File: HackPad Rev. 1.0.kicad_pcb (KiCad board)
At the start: 2 copper layers, 87 x 56.5 mm, 14 parts, among them SW1 SW_Push_45deg, SW2 SW_Push_45deg, SW3 SW_Push_45deg, SW4 SW_Push_45deg, SW5 RotaryEncoder_Switch, SW6 SW_Push_45deg, U1 Seeed Studio XIAO SAMD21

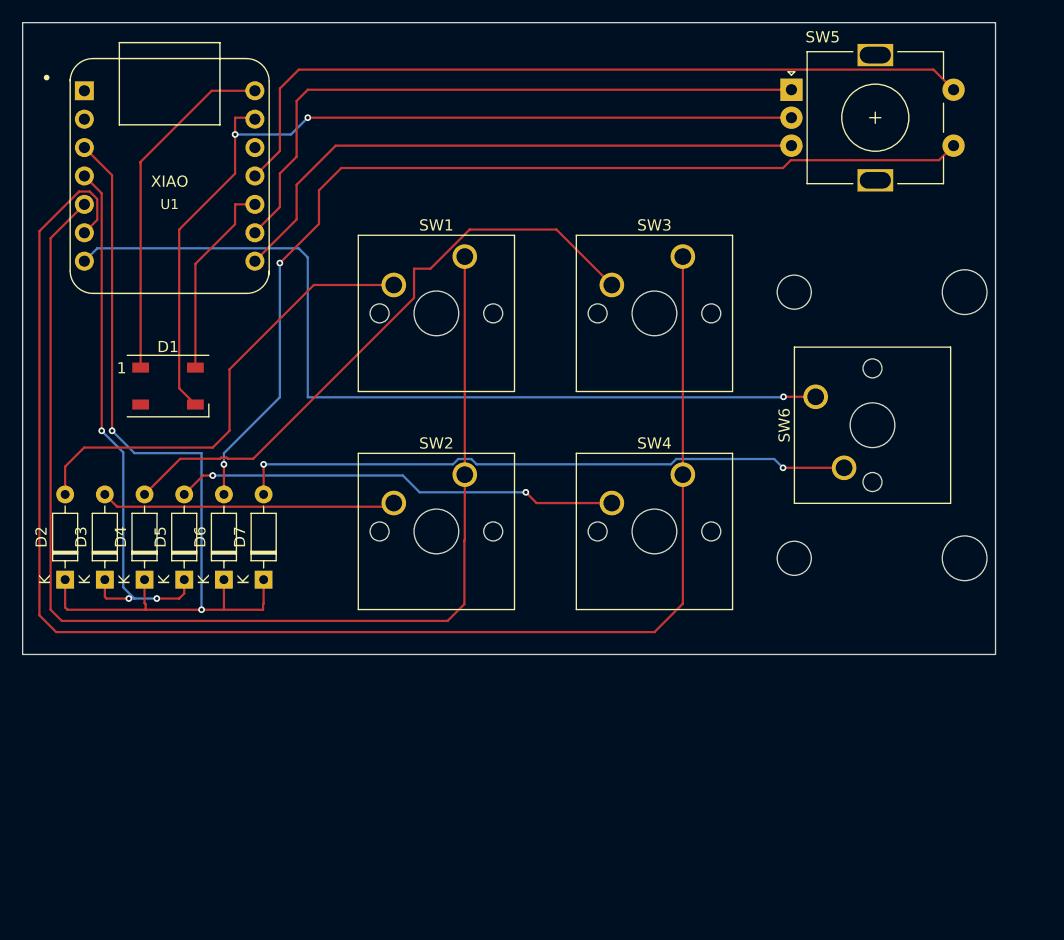
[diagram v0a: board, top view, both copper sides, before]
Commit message: finished PCB
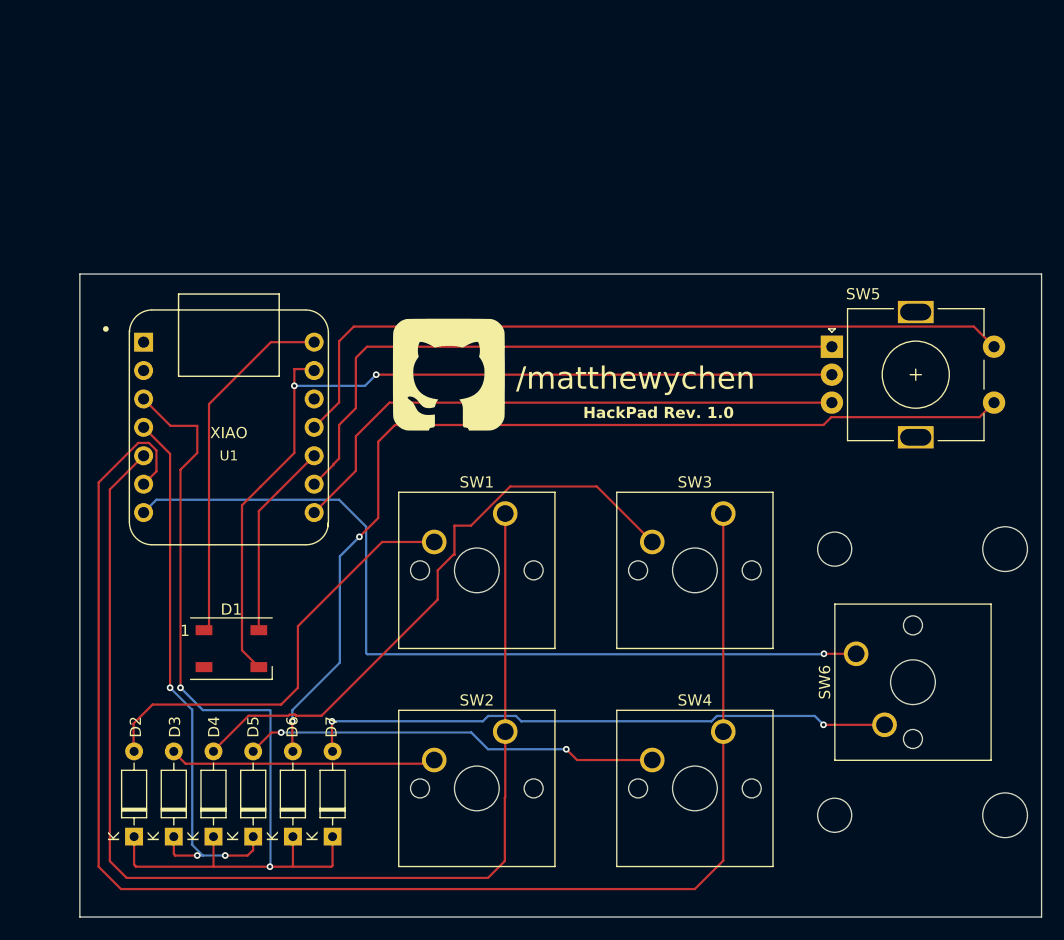
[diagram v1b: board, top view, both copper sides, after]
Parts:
- added G***: LOGO, footprints:GH LOGO, F.Cu at (133.1, 77.5)
- moved D1 24.2 mm to (113.7, 102.0)
- moved D2 23.8 mm to (105.0, 118.8)
- moved D3 23.8 mm to (108.5, 118.8)
- moved D5 23.8 mm to (115.6, 118.8)
- moved D6 23.8 mm to (119.2, 118.8)
- moved D7 23.8 mm to (122.7, 118.8)
- moved D4 23.8 mm to (112.1, 118.8)
- moved SW1 23.3 mm to (138.2, 89.9)
- moved SW2 23.3 mm to (138.2, 109.4)
- moved SW3 23.3 mm to (157.7, 89.9)
- moved SW4 23.3 mm to (157.7, 109.4)
- moved SW6 23.3 mm to (169.5, 102.4)
- moved SW5 23.3 mm to (167.4, 75.0)
- moved U1 23.1 mm to (113.4, 82.2)
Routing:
- net Net-(D2-K): track 77.6 -> 81.1 mm
- net Net-(D3-A): track 26.4 -> 23.9 mm
- net Net-(D7-A): track 55.5 -> 53.0 mm
- net Net-(D5-A): track 40.0 -> 37.5 mm
- net Net-(D2-A): track 41.8 -> 39.3 mm
- net Net-(U1-PB08_A6_D6_TX): track 78.7 -> 76.6 mm
- net Net-(U1-PA7_A8_D8_SCK): track 58.0 -> 55.9 mm
- net Net-(U1-PA6_A10_D10_MOSI): track 70.4 -> 68.5 mm
- net Net-(U1-PB09_A7_D7_RX): track 54.1 -> 52.2 mm
- net Net-(D6-A): track 89.1 -> 87.4 mm
- net /C2: track 135.0 -> 133.5 mm
- net /C0: track 106.6 -> 105.2 mm
- net GND: track 80.5 -> 79.5 mm
- net Net-(D4-A): track 55.3 -> 54.3 mm
- net Net-(D3-K): track 49.8 -> 50.6 mm
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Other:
- board size 87 x 56.5 mm -> 86 x 57.5 mm
- board text added: "/matthewychen"
- board text added: "HackPad Rev. 1.0"
